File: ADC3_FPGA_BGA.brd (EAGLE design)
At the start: 40 x 40 mm, 80 parts, among them CON1 MEZZANINE_2X30, CON2 MEZZANINE_2X30, CON3 USB-SC, IC1 3.3V, IC2 MPM3804, IC3 1.0V, IC4 LFD2NX-40, IC5 EEPROM, IC6 93LC56, IC7 FT2232H, IC8 HyperRAM, J1 CLK, X1 25MHz, X2 12MHz

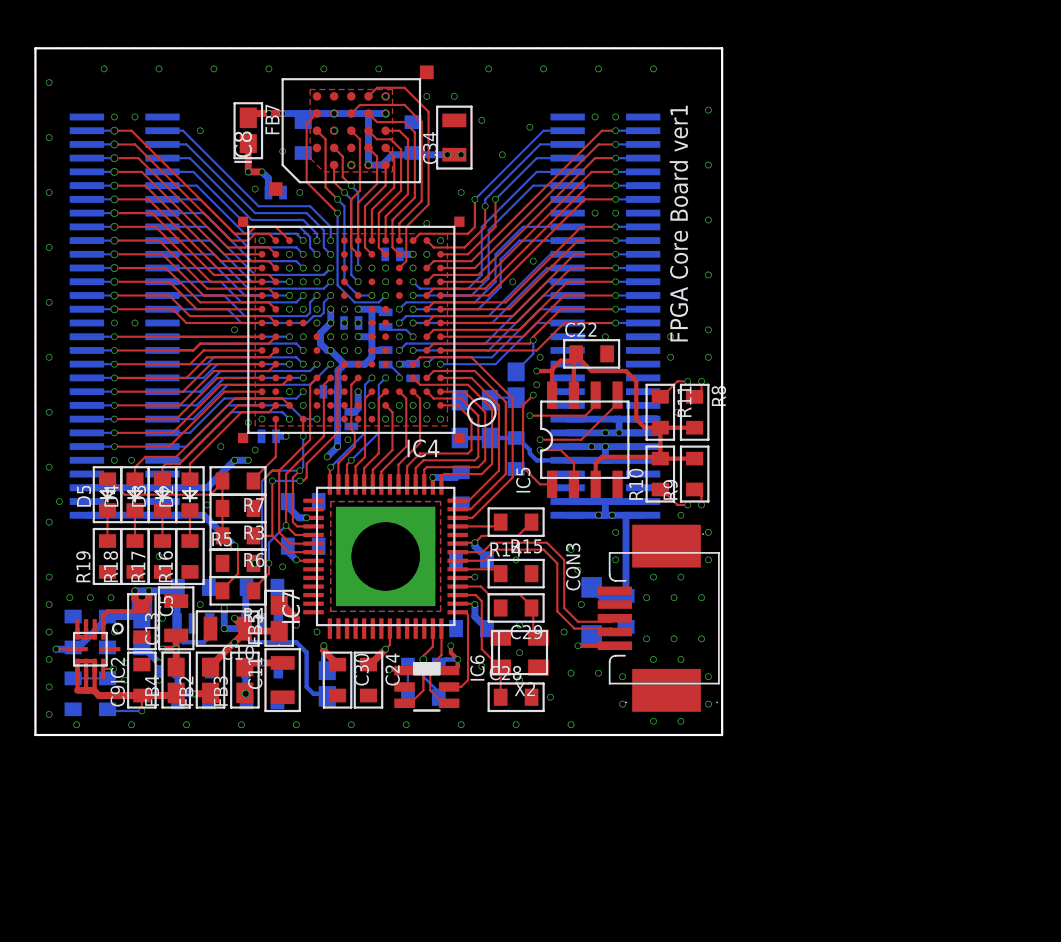
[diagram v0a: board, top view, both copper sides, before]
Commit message: Artix-7 途中
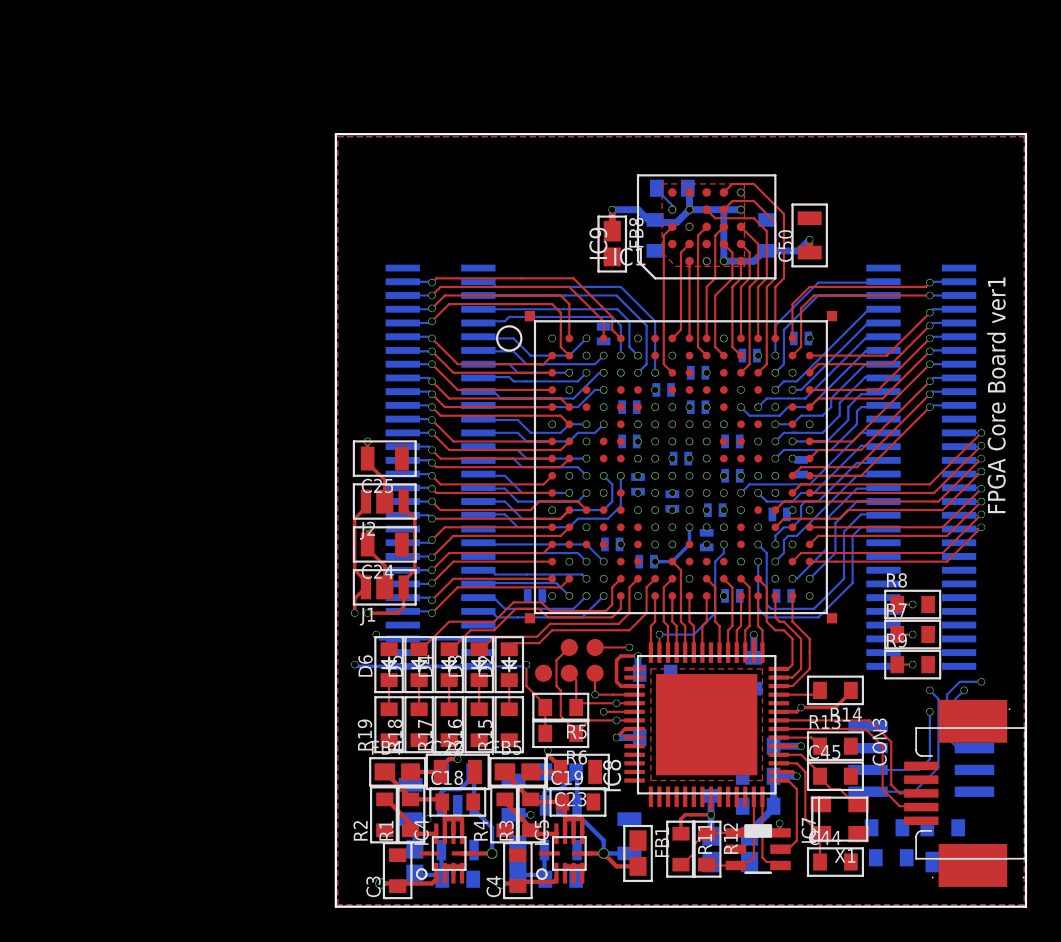
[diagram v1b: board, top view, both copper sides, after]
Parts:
- removed X2: 12MHz, my_rcl:KC3225
- added C36, C37, C38: 1u, my_rcl:1005
- added C39, C41, C42, C43, C47, C48, C49, C51: 0.1u, my_rcl:1608
- added C40, C46: 10u, my_rcl:1608
- added C44, C45: 22p, my_rcl:1608
- added C50: 10u, my_rcl:2012
- added D6: PWR, my_rcl:D1608
- added FB8: DRAM, my_rcl:1608-J
- added IC9: HyperRAM, my_ic:TFBGA24
- added J2: BANK35, my_rcl:2012-3-J
- added R20: 1k, my_rcl:1608
- added TP1: TMS, my_connector:TESTPAD
- added TP2: TDI, my_connector:TESTPAD
- added TP3: TCK, my_connector:TESTPAD
- added TP4: TDO, my_connector:TESTPAD
- added TP5: GND, my_connector:TESTPAD
- C10, C11, C13, C34: value 10u -> 1u; device my_rcl:2012 -> my_rcl:1005
- C12, C14, C15: value 0.1u -> 1u
- C16, C17, C18: value 0.1u -> 10u; device my_rcl:1005 -> my_rcl:1608
- C19, C4: value 0.1u -> 10u
- C2, C24: device my_rcl:1608 -> my_rcl:2012
- C20, C21, C23: value 0.1u -> 10u; device my_rcl:1005 -> my_rcl:2012
- C22, C25: value 0.1u -> 10u; device my_rcl:1608 -> my_rcl:2012
- C26, C27, C31, C32, C33, C35: value 0.1u -> 1u; device my_rcl:1608 -> my_rcl:1005
- C28, C29: value 22p -> 1u; device my_rcl:1608 -> my_rcl:1005
- C30, C9: value 10u -> 1u; device my_rcl:1608 -> my_rcl:1005
- C5: value 10u -> 0.1u
- C7, C8: device my_rcl:1608 -> my_rcl:1005
- D5: value PWR -> LED2
- FB3, IC3: value 1.0V -> 2.5V
- FB5: value FT -> 1.0V
- FB7: value DRAM -> FT
- IC1: value 3.3V -> ARTIX7-FTG256; device my_ic:SOT23-5 -> my_ic:FTG256
- IC2: value MPM3804 -> 3.3V; device my_ic:QFN-10 -> my_ic:SOT23-5
- IC4: value LFD2NX-40 -> MPM3804; device my_ic:CABGA192 -> my_ic:QFN-10
- IC5: value EEPROM -> MPM3804; device my_ic:SOP8 -> my_ic:QFN-10
- IC6: value 93LC56 -> EEPROM; device my_ic:SOT23-6 -> my_ic:SOIC-SOIJ-8
- IC7: value FT2232H -> 93LC56; device my_ic:VQFN56 -> my_ic:SOT23-6
- IC8: value HyperRAM -> FT2232H-2; device my_ic:TFBGA24 -> my_ic:QFN56-HT
- J1: value CLK -> BANK34; device my_rcl:1608-J -> my_rcl:2012-3-J
- R12, R3: value 10k -> 1k
- R13: value 1k -> 12.1k
- R14: value 12.1k -> 1k
- R4: value 10k -> 1.5k
- X1: value 25MHz -> 12MHz
- moved FB7 51.0 mm to (4.00, -22.2), flipped to the bottom, turned to 90 degrees
- moved IC8 40.3 mm to (1.50, -15.0)
- moved R7 40.3 mm to (13.5, -9.75), turned to 0 degrees
- moved C16 37.7 mm to (-7.00, -24.0), turned to 180 degrees
- moved C18 37.0 mm to (-13.0, -19.5), flipped to the top, turned to 0 degrees
- moved C9 36.1 mm to (1.00, 3.50), flipped to the bottom, turned to 0 degrees
- moved C35 34.8 mm to (7.00, 0.00)
- moved C2 32.6 mm to (-3.00, -21.5), turned to 90 degrees
- moved FB1 31.6 mm to (-2.50, -22.5), flipped to the top, turned to 270 degrees
- moved X1 31.5 mm to (9.25, -20.5), flipped to the top, turned to 0 degrees
- moved C10 31.2 mm to (1.00, 5.50), flipped to the bottom, turned to 0 degrees
- moved IC4 31.0 mm to (-13.5, -22.5), turned to 90 degrees
- moved C13 30.8 mm to (0.00, 0.50), flipped to the bottom, turned to 0 degrees
- moved C31 30.5 mm to (7.00, 7.50), turned to 0 degrees
- moved C8 30.4 mm to (3.00, -0.50), turned to 0 degrees
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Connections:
- removed net +1V0_LDO: C8.1, FB3.1, IC3.5
- removed net +3.3V_LDO: C7.1, FB2.1, IC1.5
- removed net ADC_DN1: CON1.30, IC4.H14
- removed net ADC_DP1: CON1.28, IC4.H13
- removed net INITN: IC4.B2, R8.1
- removed net JTAG_EN: IC4.A13, R7.1
- removed net N$6: J1.1, X1.3
- removed net N$7: IC2.9, R1.1, R2.2
- removed net PB10A: CON2.7, IC4.L2
- removed net PB10B: CON2.3, IC4.M2
- removed net PB12A: CON2.6, IC4.P2
- removed net PB12B: CON2.4, IC4.P3
- removed net PB4A: CON2.13, IC4.K1
- removed net PB4B: CON2.9, IC4.L1
- removed net PB58A: CON1.3, IC4.P9
- removed net PB58B: CON1.5, IC4.N9
- removed net PB60A: CON1.7, IC4.P10
- removed net PB60B: CON1.9, IC4.N10
- removed net PB64A: CON1.17, IC4.M9
- removed net PB64B: CON1.21, IC4.L9
- removed net PB66A: CON1.29, IC4.K9
- removed net PB66B: CON1.27, IC4.K10
- removed net PB68A: CON1.15, IC4.M11
- removed net PB68B: CON1.19, IC4.L12
- removed net PB6A: CON2.12, IC4.K3
- removed net PB6B: CON2.10, IC4.L3
- removed net PB70A: CON1.25, IC4.K11
- removed net PB70B: CON1.23, IC4.K12
- removed net PB72A: CON1.11, IC4.P11
- removed net PB72B: CON1.13, IC4.N11
- removed net PB74A: CON1.4, IC4.P12
- removed net PB74B: CON1.6, IC4.P13
- removed net PB76A: CON1.8, IC4.N13
- removed net PB76B: CON1.10, IC4.N14
- removed net PB78A: CON1.14, IC4.M14
- removed net PB78B: CON1.12, IC4.M13
- removed net PB80A: CON1.16, IC4.L13
- removed net PB80B: CON1.18, IC4.L14
- removed net PB82A: CON1.20, IC4.K13
- removed net PB82B: CON1.22, IC4.K14
- removed net PB84A: CON1.26, IC4.J14
- removed net PB84B: CON1.24, IC4.J13
- removed net PB8A: CON2.5, IC4.M1
- removed net PB8B: CON2.8, IC4.N1
- removed net PL24A: CON2.30, IC4.E2
- removed net PL24B: CON2.32, IC4.E1
- removed net PL26A: CON2.28, IC4.F3
- removed net PL26B: CON2.26, IC4.F4
- removed net PL30A: CON2.29, IC4.F2, J1.2
- removed net PL30B: CON2.31, IC4.F1
- removed net PL32A: CON2.27, IC4.G1
- removed net PL32B: CON2.25, IC4.G2
- removed net PL36A: CON2.23, IC4.H1
- removed net PL36B: CON2.21, IC4.H2
- removed net PL38A: CON2.24, IC4.H3
- removed net PL38B: CON2.22, IC4.H4
- removed net PL42A: CON2.19, IC4.J1
- removed net PL42B: CON2.17, IC4.J2
- removed net PL44A: CON2.20, IC4.J3
- removed net PL44B: CON2.18, IC4.J4
- removed net PL47A: CON2.11, IC4.K2
- removed net PR13B: CON1.51, IC4.A12
- removed net PR17A: CON1.49, IC4.A10
- removed net PR24A: CON1.46, IC4.D14
- removed net PR24B: CON1.50, IC4.C14
- removed net PR26A: CON1.47, IC4.C11
- removed net PR27A: CON1.48, IC4.D12
- removed net PR27B: CON1.39, IC4.E12
- removed net PR30A: CON1.45, IC4.E9
- removed net PR30B: CON1.41, IC4.E10
- removed net PR32A: CON1.43, IC4.D11
- removed net PR32B: CON1.37, IC4.E11
- removed net PR34A: CON1.40, IC4.F13
- removed net PR34B: CON1.38, IC4.F14
- removed net PR36A: CON1.44, IC4.E13
- removed net PR36B: CON1.42, IC4.E14
- removed net PR38A: CON1.34, IC4.G14
- removed net PR38B: CON1.36, IC4.G13
- removed net PR42A: CON1.35, IC4.F11
- removed net PR42B: CON1.33, IC4.G12
- removed net PROGRAMN: IC4.A2, R9.1
- new net +1V0_DCDC: C19.1, FB5.1, IC5.6, IC5.7, IC5.8, R3.2
- new net +1V0_DCDC_FB: IC5.9, R3.1, R4.2
- new net +1V8_DCDC_FB: IC4.9, R1.1, R2.2
- new net +2V5: C21.1, CON2.49, CON2.50, FB3.2, J1.3, J2.3
- new net +2V5_LDO: C17.1, FB3.1, IC3.5
- new net +3V3_LDO: C16.1, FB2.1, IC2.5
- new net 1.0V_DCDC_SW: IC5.2, IC5.3, IC5.4
- new net INIT_B: IC1.K10, R7.1
- new net IO0_14: CON2.26, IC1.K12
- new net IO10N_15: CON2.7, IC1.B16
- new net IO10N_35: CON1.16, IC1.D1
- new net IO10P_15: CON2.9, IC1.C16
- new net IO10P_35: CON1.18, IC1.E2
- new net IO11N_14: CON2.40, IC1.P13
- new net IO11P_14: CON2.38, IC1.N13
- new net IO12N_14: CON2.32, IC1.P14
- new net IO12N_35: CON1.19, IC1.C4
- new net IO12P_14: CON2.30, IC1.N14
- new net IO12P_35: CON1.21, IC1.D4
- new net IO13N_15: CON2.12, IC1.E13
- new net IO13P_15: CON2.14, IC1.E12
- new net IO14N_35: CON1.23, IC1.F3
- new net IO14P_35: CON1.25, IC1.F4
- new net IO15N_15: CON2.10, IC1.D15
- new net IO15N_35: CON1.20, IC1.E1
- new net IO15P_15: CON2.8, IC1.D14
- new net IO15P_35: CON1.22, IC1.F2
- new net IO17N_15: CON2.11, IC1.D16
- new net IO17N_35: CON1.24, IC1.G1
- new net IO17P_15: CON2.13, IC1.E16
- new net IO17P_35: CON1.26, IC1.G2
- new net IO19N_35: CON1.35, IC1.J4
- new net IO19P_35: CON1.37, IC1.J5
- new net IO20N_35: CON1.28, IC1.H1
- new net IO20P_35: CON1.30, IC1.H2
- new net IO21N_15: CON2.16, IC1.F14
- new net IO21N_35: CON1.27, IC1.H3
- new net IO21P_15: CON2.18, IC1.G14
- new net IO21P_35: CON1.29, IC1.J3
- new net IO22N_15: CON2.15, IC1.G16
- new net IO22N_35: CON1.32, IC1.J1
- new net IO22P_15: CON2.17, IC1.H16
- new net IO22P_35: CON1.34, IC1.K1
- new net IO23N_15: CON2.21, IC1.J16
- new net IO23N_35: CON1.38, IC1.L2
- new net IO23P_15: CON2.19, IC1.J15
- new net IO23P_35: CON1.36, IC1.L3
- new net IO24N_15: CON2.20, IC1.G15
- new net IO24N_35: CON1.31, IC1.K2
- new net IO24P_15: CON2.22, IC1.H14
- new net IO24P_35: CON1.33, IC1.K3
- new net IO2N_14: CON2.27, IC1.K16
- new net IO2N_34: CON1.42, IC1.M1
- new net IO2N_35: CON1.9, IC1.B5
- new net IO2P_14: CON2.25, IC1.K15
- new net IO2P_34: CON1.44, IC1.M2
- new net IO2P_35: CON1.7, IC1.B6
- new net IO3N_35: CON1.6, IC1.A4
- new net IO3P_35: CON1.4, IC1.A5
- new net IO4N_14: CON2.31, IC1.M14
- new net IO4N_34: CON1.48, IC1.P1
- new net IO4N_35: CON1.11, IC1.A3
- new net IO4P_14: CON2.29, IC1.L14
- new net IO4P_34: CON1.46, IC1.N1
- new net IO4P_35: CON1.13, IC1.B4
- new net IO5N_34: CON1.43, IC1.P3
- new net IO5N_35: CON1.5, IC1.C6
- new net IO5P_14: CON2.28, IC1.K13
- new net IO5P_34: CON1.41, IC1.P4
- new net IO5P_35: CON1.3, IC1.C7
- new net IO7N_14: CON2.35, IC1.N16
- new net IO7N_34: CON1.50, IC1.R1
- new net IO7N_35: CON1.15, IC1.C2
- new net IO7P_14: CON2.33, IC1.M16
- new net IO7P_34: CON1.52, IC1.R2
- new net IO7P_35: CON1.17, IC1.C3
- new net IO8N_14: CON2.39, IC1.P16
- new net IO8N_15: CON2.4, IC1.B14
- new net IO8N_34: CON1.47, IC1.T2
- new net IO8N_35: CON1.8, IC1.A2
- new net IO8P_14: CON2.37, IC1.P15
- new net IO8P_15: CON2.6, IC1.C14
- new net IO8P_34: CON1.45, IC1.R3
- new net IO8P_35: CON1.10, IC1.B2
- new net IO9N_14: CON2.36, IC1.R16
- new net IO9N_15: CON2.3, IC1.A15
- new net IO9N_34: CON1.49, IC1.T3
- new net IO9N_35: CON1.12, IC1.B1
- new net IO9P_14: CON2.34, IC1.R15
- new net IO9P_15: CON2.5, IC1.B15
- new net IO9P_34: CON1.51, IC1.T4
- new net IO9P_35: CON1.14, IC1.C1
- new net LED3: D5.A, IC1.R5
- new net N$5: D5.K, R18.2
- new net PROGRAM_B: IC1.L9, R8.1
- new net VCCO34: C24.1, C26.1, C28.1, IC1.M3, IC1.R4, IC1.T1, J1.2
- new net VCCO35: C25.1, C27.1, C29.1, C30.1, IC1.A6, IC1.B3, IC1.D7, IC1.E4, IC1.F1, IC1.J2, J2.2
- net +1V0: now also C13.1, C23.1, C7.1, C9.1, FB5.2, IC1.E10, IC1.F11, IC1.F7, IC1.F9, IC1.G6, IC1.H9, IC1.J6, IC1.K9, IC1.L8; no longer C12.1, C17.1, FB3.2, IC4.F9, IC4.G7, IC4.H9, IC4.J7, IC4.J9
- net +1V8: now also C10.1, C12.1, C22.1, C31.1, C33.1, C35.1, C8.1, FB7.1, FB8.2, IC1.A16, IC1.B13, IC1.C10, IC1.E14, IC1.G10, IC1.G8, IC1.H15, IC1.J10, IC1.J12, IC1.K11, IC1.L10; no longer C13.1, C16.1, C18.1, C23.1, C6.1, FB6.1, FB7.2, IC3.1, IC3.3, IC4.F7, IC4.G9, IC4.H10, IC4.H7, IC4.J10, IC4.J12, IC4.L11, IC4.L5, IC4.M10, IC4.M3, IC4.M6, IC4.N12, IC4.N3
- net +1V8_DCDC: now also C18.1, IC4.6, IC4.7, IC4.8; no longer C9.1, IC2.6, IC2.7, IC2.8
- net +3V3: now also C32.1, C34.1, C36.1, C37.1, C38.1, C39.1, D6.A, FB6.1, IC1.E7, IC1.L15, IC1.L16, IC1.L6, IC1.M13, IC1.M9, IC1.N10, IC1.P7, IC1.R14, IC1.T11, IC6.3, IC6.7, IC6.8, J1.1, J2.1, R5.2; no longer C10.1, C19.1, C21.1, C22.1, CON2.49, CON2.50, D5.A, FB5.1, IC4.C12, IC4.C7, IC4.E4, IC4.G11, IC4.G4, IC5.3, IC5.7, IC5.8, R11.2, R3.2, R4.2, X1.1, X1.4
- net 1.8V_DCDC_SW: now also IC4.2, IC4.3, IC4.4; no longer IC2.2, IC2.3, IC2.4
- net DONE: now also IC1.H10, R9.1; no longer IC4.A3, R10.1
- net DRAM_+1V8: now also C49.1, C50.1, C51.1, FB8.1, IC9.B4, IC9.D1, IC9.E4, R20.2; no longer C33.1, C34.1, C35.1, FB7.1, IC8.B4, IC8.D1, IC8.E4
- net DRAM_CKN: now also IC1.A9, IC9.B1; no longer IC4.L7, IC8.B1
- net DRAM_CKP: now also IC1.A8, IC9.B2; no longer IC4.M7, IC8.B2
- net DRAM_CS: now also IC1.C8, IC9.A3; no longer IC4.K6, IC8.A3
- net DRAM_DQ0: now also IC1.A10, IC9.D3; no longer IC4.N5, IC8.D3
- net DRAM_DQ1: now also IC1.B11, IC9.D2; no longer IC4.P7, IC8.D2
- net DRAM_DQ2: now also IC1.A13, IC9.C4; no longer IC4.P4, IC8.C4
- net DRAM_DQ3: now also IC1.C13, IC9.D4; no longer IC4.N4, IC8.D4
- net DRAM_DQ4: now also IC1.A14, IC9.D5; no longer IC4.M4, IC8.D5
- net DRAM_DQ5: now also IC1.C12, IC9.E3; no longer IC4.P5, IC8.E3
- net DRAM_DQ6: now also IC1.A12, IC9.E2; no longer IC4.P6, IC8.E2
- net DRAM_DQ7: now also IC1.B12, IC9.E1; no longer IC4.N6, IC8.E1
- net DRAM_NRST: now also IC9.A4, R20.1; no longer IC4.K5, IC8.A4
- net DRAM_RWDS: now also IC1.B10, IC9.C3; no longer IC4.N7, IC8.C3
- net FLASH_CS: now also IC1.L12, IC6.1, R10.1; no longer IC4.B4, IC5.1, R11.1
- net FLASH_MISO: now also IC1.J14, IC6.2; no longer IC4.A5, IC5.2
- net FLASH_MOSI: now also IC1.J13, IC6.5; no longer IC4.A4, IC5.5
- net FLASH_SCK: now also IC1.E8, IC6.6; no longer IC4.B3, IC5.6
- net FT_+1V8: now also C46.1, C47.1, C48.1, FB7.2, IC8.2, IC8.31; no longer C30.1, C31.1, C32.1, FB6.2, IC7.2, IC7.31
- net FT_+3V3: now also C40.1, C41.1, C42.1, C43.1, FB6.2, IC7.6, IC8.16, IC8.36, IC8.5, IC8.50, IC8.9, R11.1, R14.1; no longer C24.1, C25.1, C26.1, C27.1, FB5.2, IC6.6, IC7.16, IC7.36, IC7.5, IC7.50, IC7.9, R12.1, R15.1
- net FT_CLK: now also IC1.N11, IC8.27; no longer IC4.D7, IC7.27
- net FT_D0: now also IC1.T15, IC8.12; no longer IC4.E3, IC7.12
- net FT_D1: now also IC1.T14, IC8.13; no longer IC4.D2, IC7.13
- net FT_D2: now also IC1.R13, IC8.14; no longer IC4.D1, IC7.14
- net FT_D3: now also IC1.T13, IC8.15; no longer IC4.D3, IC7.15
- net FT_D4: now also IC1.R12, IC8.17; no longer IC4.C1, IC7.17
- net FT_D5: now also IC1.T12, IC8.18; no longer IC4.C2, IC7.18
- net FT_D6: now also IC1.R11, IC8.19; no longer IC4.B1, IC7.19
- net FT_D7: now also IC1.R10, IC8.20; no longer IC4.C3, IC7.20
- net FT_NOE: now also IC1.T7, IC8.28; no longer IC4.D6, IC7.28
- net FT_NRD: now also IC1.P8, IC8.24; no longer IC4.C5, IC7.24
- net FT_NWR: now also IC1.T8, IC8.25; no longer IC4.C6, IC7.25
- net FT_RXNF: now also IC1.T10, IC8.22; no longer IC4.C4, IC7.22
- net FT_SIWU: now also IC1.R8, IC8.26; no longer IC4.D5, IC7.26
- net FT_TXNE: now also IC1.T9, IC8.23; no longer IC4.B5, IC7.23
- net GND: now also C36.2, C37.2, C38.2, C39.2, C40.2, C41.2, C42.2, C43.2, C44.2, C45.2, C46.2, C47.2, C48.2, C49.2, C50.2, C51.2, CON1.39, CON1.40, CON2.23, CON2.24, IC1.A1, IC1.A11, IC1.B8, IC1.C15, IC1.C5, IC1.D12, IC1.D2, IC1.E9, IC1.F10, IC1.F16, IC1.F6, IC1.F8, IC1.G13, IC1.G3, IC1.G7, IC1.G9, IC1.H6, IC1.H7, IC1.H8, IC1.J11, IC1.J7, IC1.J8, IC1.J9, IC1.K14, IC1.K4, IC1.K6, IC1.K7, IC1.K8, IC1.L1, IC1.L11, IC1.M10, IC1.M11, IC1.M8, IC1.N15, IC1.N5, IC1.P12, IC1.P2, IC1.R9, IC1.T16, IC1.T6, IC2.2, IC4.10, IC5.10, IC6.4, IC7.2, IC8.10, IC8.21, IC8.41, IC8.45, IC8.HT, IC9.B3, IC9.C1, IC9.E5, R13.2, R15.1, R4.1, TP5.1, X1.4; no longer CON1.31, CON1.32, CON1.52, CON2.14, CON2.15, CON2.16, CON2.33, CON2.34, CON2.35, CON2.36, CON2.37, CON2.38, CON2.39, CON2.40, IC1.2, IC2.10, IC4.A1, IC4.A14, IC4.B11, IC4.B6, IC4.D4, IC4.F12, IC4.F8, IC4.G3, IC4.G8, IC4.H8, IC4.J11, IC4.J8, IC4.L10, IC4.M12, IC4.M5, IC4.N2, IC4.P1, IC4.P14, IC5.4, IC6.2, IC7.10, IC7.21, IC7.41, IC7.45, IC7.HT, IC8.B3, IC8.C1, IC8.E5, R14.2, R5.1, X2.2, X2.4
- net JTAG_TCK: now also IC1.L7, IC8.32, TP3.1; no longer IC4.A11, IC7.32, R5.2
- net JTAG_TDI: now also IC1.N7, IC8.33, R5.1, TP2.1; no longer IC4.D9, IC7.33, R4.1
- net JTAG_TDO: now also IC1.N8, IC8.34, TP4.1; no longer IC4.D10, IC7.34, R3.1
- net JTAG_TMS: now also IC1.M7, IC8.35, TP1.1; no longer IC4.E8, IC7.35
- net LED0: now also IC1.R7; no longer IC4.B13
- net LED1: now also IC1.R6; no longer IC4.B14
- net LED2: now also IC1.T5; no longer IC4.B12
- net N$1: now also D6.K; no longer D5.K
- net N$10: now also IC7.3, IC8.55, R12.2; no longer IC6.3, IC7.55, R13.2
- net N$11: now also IC7.5, IC8.1; no longer IC6.5, IC7.1
- net N$12: now also IC7.1, R11.2, R12.1; no longer IC6.1, R12.2, R13.1
- net N$13: now also C45.1, IC8.4, X1.3; no longer C29.1, IC7.4, X2.3
- net N$14: now also C44.1, IC8.3, X1.1; no longer C28.1, IC7.3, X2.1
- net N$15: now also IC8.6, R13.1; no longer IC7.6, R14.1
- net N$16: now also IC8.11, R14.2; no longer IC7.11, R15.2
- net N$2: now also R15.2; no longer R16.2
- net N$3: now also R16.2; no longer R17.2
- net N$4: now also R17.2; no longer R18.2
- net N$9: now also IC7.4, IC8.56; no longer IC6.4, IC7.56
- net USB_DM: now also IC8.7; no longer IC7.7
- net USB_DP: now also IC8.8; no longer IC7.8
- net VIN_DCDC: now also C6.1, IC2.3, IC3.1, IC3.3, IC4.1, IC4.5, IC5.1, IC5.5; no longer IC1.1, IC1.3, IC2.5
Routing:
- net +1V8: track 242.0 -> 69.9 mm, vias 24 -> 13
- net +3V3: track 223.2 -> 95.1 mm, vias 11 -> 14
- net VIN: track 96.2 -> 0.00 mm, vias 4 -> 0
- net VCCO35: track 0.00 -> 32.1 mm, vias 0 -> 7
- net FT_+3V3: track 73.1 -> 44.5 mm, vias 8 -> 6
- net FLASH_SCK: track 11.7 -> 37.4 mm
- net +2V5: track 0.00 -> 25.2 mm, vias 0 -> 2
- net VCCO34: track 0.00 -> 23.7 mm, vias 0 -> 4
- net VIN_DCDC: track 24.9 -> 47.1 mm, vias 3 -> 4
- net INIT_B: track 0.00 -> 20.4 mm, vias 0 -> 2
- net PROGRAMN: track 19.9 -> 0.00 mm, vias 2 -> 0
- net PROGRAM_B: track 0.00 -> 17.8 mm, vias 0 -> 2
- net INITN: track 17.8 -> 0.00 mm, vias 2 -> 0
- net FLASH_MISO: track 13.3 -> 31.0 mm
- net FT_+1V8: track 45.7 -> 28.3 mm, vias 3 -> 2
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- removed copper zone on layer 2, net GND
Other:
- board size 40 x 40 mm -> 40.2 x 45 mm
